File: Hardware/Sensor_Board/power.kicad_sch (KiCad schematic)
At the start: 25 parts, among them U201 TPS7A20L_1V2, U202 TPS7A20L_2V2, U203 TPS7A20L_3V3, U204 TLV840, U205 ICE40UL1K-CM36AI

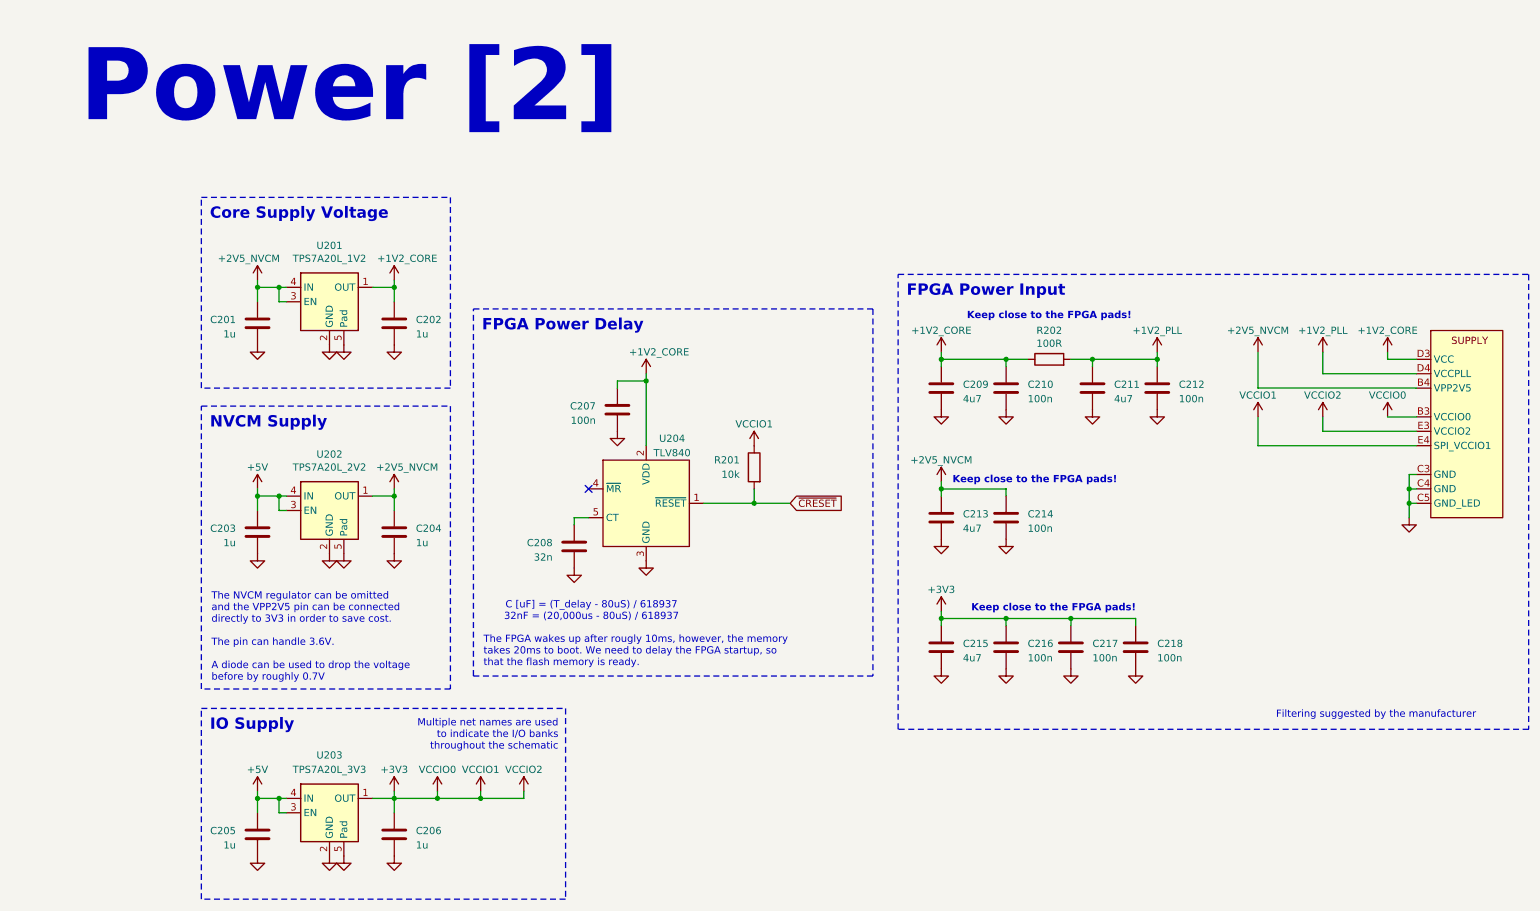
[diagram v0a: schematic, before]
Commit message: Cleared ERC errors and improved folder structure
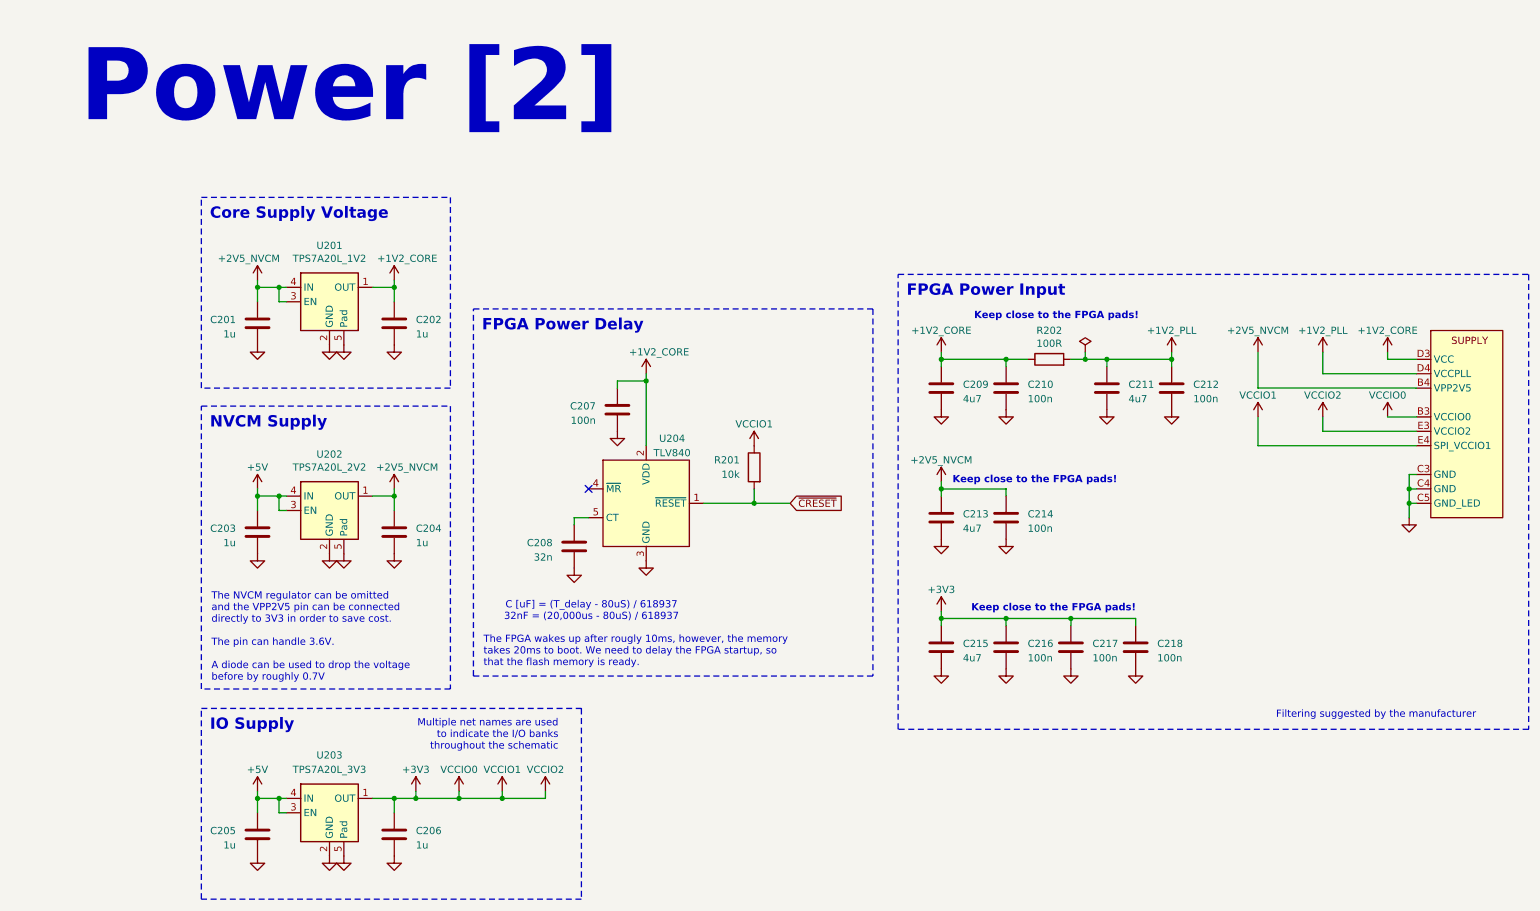
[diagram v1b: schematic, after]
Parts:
- removed U205: ICE40UL1K-CM36AI, Package_BGA:UCBGA-36_2.5x2.5mm_Layout6x6_P0.4mm, symbol Custom_VoxLink_Symbols:ICE40UL1K-CM36AI
- added U301: ICE40UL1K-CM36AI, Package_BGA:UCBGA-36_2.5x2.5mm_Layout6x6_P0.4mm, symbol Custom_VoxLink_Symbols:ICE40UL1K-CM36AI
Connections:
- net +1V2_CORE: now also U301.D3 (VCC)
- net +1V2_PLL: now also U301.D4 (VCCPLL)
- net +2V5_NVCM: now also U301.B4 (VPP2V5)
- net +3V3: now also U301.B3 (VCCIO0), U301.E3 (VCCIO2), U301.E4 (SPI_VCCIO1)
- net GND: now also U301.C3 (GND), U301.C4 (GND), U301.C5 (GND_LED)
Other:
- moved on the sheet: C211, C212
